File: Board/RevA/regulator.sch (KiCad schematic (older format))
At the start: 0 parts

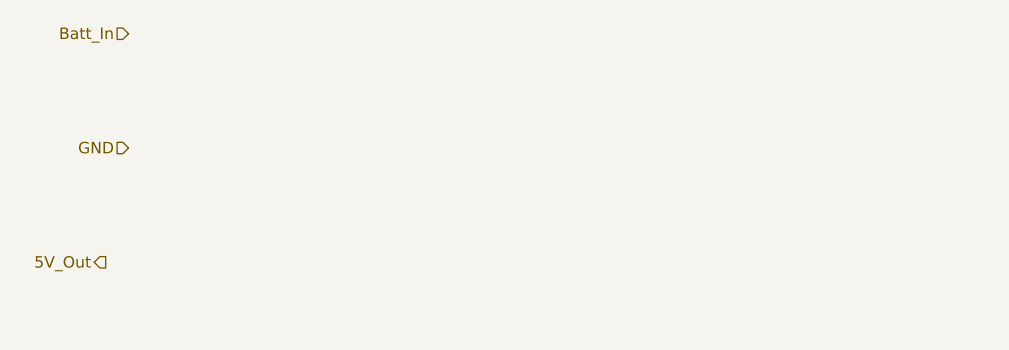
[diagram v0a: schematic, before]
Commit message: Finished Rough RevA and Added Annotations
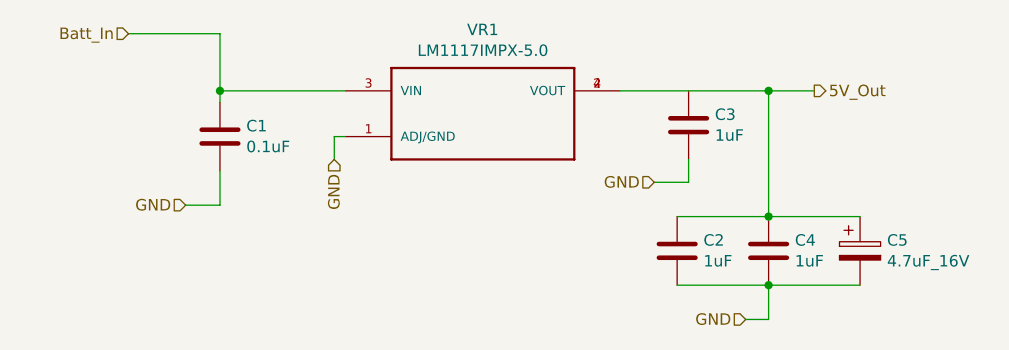
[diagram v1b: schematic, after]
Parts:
- added C1: 0.1uF, symbol Device:C
- added C2, C3, C4: 1uF, symbol Device:C
- added C5: 4.7uF_16V, symbol Device:CP
- added VR1: LM1117IMPX-5.0, symbol LM1117IMPX-5.0:LM1117IMPX-5.0
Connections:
- net 5V_Out: now also C2.1, C4.1, C5.1, VR1.2 (VOUT), VR1.4 (VOUT)
- net Batt_In: now also C1.1, VR1.3 (VIN)
- net GND: now also C1.2, C2.2, C3.2, C4.2, C5.2, VR1.1 (ADJ/GND)
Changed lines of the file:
@@
 Text HLabel 3400 2700 0    50   Input ~ 0
 Batt_In
-Text HLabel 3400 3200 0    50   Input ~ 0
+Text HLabel 3650 3450 0    50   Input ~ 0
 GND
-Text HLabel 3300 3700 0    50   Output ~ 0
+Text HLabel 6400 2950 2    50   Output ~ 0
 5V_Out
+$Comp
+L LM1117IMPX-5.0:LM1117IMPX-5.0 VR1
+U 1 1 614A1D39
+P 4950 3050
+F 0 "VR1" H 4950 3417 50  0000 C CNN
+F 1 "LM1117IMPX-5.0" H 4950 3326 50  0000 C CNN
+F 2 "" H 4950 3050 50  0001 L BNN
+F 3 "1.80 mm" H 4950 3050 50  0001 L BNN
+F 4 "O" H 4950 3050 50  0001 L BNN "Field4"
+F 5 "IPC 7351B" H 4950 3050 50  0001 L BNN "Field5"
+F 6 "Rochester Electronics/Texas Instruments" H 4950 3050 50  0001 L BNN "Field6"
+	1    4950 3050
+	1    0    0    -1
+$EndComp
+$Comp
+L Device:C C1
+U 1 1 614A34B9
+P 3800 3150
+F 0 "C1" H 3915 3196 50  0000 L CNN
+F 1 "0.1uF" H 3915 3105 50  0000 L CNN
+F 2 "" H 3838 3000 50  0001 C CNN
+F 3 "~" H 3800 3150 50  0001 C CNN
+	1    3800 3150
+	1    0    0    -1
+$EndComp
+$Comp
+L Device:C C4
+U 1 1 614A3F1C
+P 6200 3650
+F 0 "C4" H 6315 3696 50  0000 L CNN
+F 1 "1uF" H 6315 3605 50  0000 L CNN
+F 2 "" H 6238 3500 50  0001 C CNN
+F 3 "~" H 6200 3650 50  0001 C CNN
+	1    6200 3650
+	1    0    0    -1
+$EndComp
+Wire Wire Line
+	4350 2950 3800 2950
+Wire Wire Line
+	3800 2950 3800 3000
+Wire Wire Line
+	3800 2950 3800 2700
+Wire Wire Line
+	3800 2700 3400 2700
+Connection ~ 3800 2950
+Wire Wire Line
+	3800 3300 3800 3450
+Wire Wire Line
+	3800 3450 3650 3450
+Wire Wire Line
+	6400 2950 6200 2950
+$Comp
+L Device:C C3
+U 1 1 614A7535
+P 5850 3100
+F 0 "C3" H 5965 3146 50  0000 L CNN
+F 1 "1uF" H 5965 3055 50  0000 L CNN
+F 2 "" H 5888 2950 50  0001 C CNN
+F 3 "~" H 5850 3100 50  0001 C CNN
+	1    5850 3100
+	1    0    0    -1
+$EndComp
+$Comp
+L Device:C C2
+U 1 1 614A7ADA
+P 5800 3650
+F 0 "C2" H 5915 3696 50  0000 L CNN
+F 1 "1uF" H 5915 3605 50  0000 L CNN
+F 2 "" H 5838 3500 50  0001 C CNN
+F 3 "~" H 5800 3650 50  0001 C CNN
+	1    5800 3650
+	1    0    0    -1
+$EndComp
+$Comp
+L Device:CP C5
+U 1 1 614A9413
+P 6600 3650
+F 0 "C5" H 6718 3696 50  0000 L CNN
+F 1 "4.7uF_16V" H 6718 3605 50  0000 L CNN
+F 2 "" H 6638 3500 50  0001 C CNN
+F 3 "~" H 6600 3650 50  0001 C CNN
+	1    6600 3650
+	1    0    0    -1
+$EndComp
+Wire Wire Line
+	6600 3500 6200 3500
+Wire Wire Line
+	6200 3500 5800 3500
+Connection ~ 6200 3500
+Wire Wire Line
+	5800 3800 6200 3800
+Wire Wire Line
+	6600 3800 6200 3800
+Connection ~ 6200 3800
+Wire Wire Line
+	6200 3500 6200 2950
+Connection ~ 6200 2950
+Wire Wire Line
+	6200 2950 5550 2950
+Text HLabel 5700 3350 0    50   Input ~ 0
+GND
+Text HLabel 6100 3950 0    50   Input ~ 0
+GND
+Wire Wire Line
+	6100 3950 6200 3950
+Wire Wire Line
+	6200 3950 6200 3800
+Wire Wire Line
+	5700 3350 5850 3350
+Wire Wire Line
+	5850 3350 5850 3250
+Text HLabel 4300 3250 3    50   Input ~ 0
+GND
+Wire Wire Line
+	4300 3250 4300 3150
+Wire Wire Line
+	4300 3150 4350 3150
 $EndSCHEMATC

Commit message: Added Footprints to RevA 1/2
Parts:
- C1, C2, C3, C4: footprint (none) -> Capacitor_SMD:C_0603_1608Metric
- C5: footprint (none) -> Capacitor_Tantalum_SMD:CP_EIA-3216-18_Kemet-A
- VR1: footprint (none) -> LM1117IMPX-5:SOT230P700X180-4N
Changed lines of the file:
@@
 F 0 "VR1" H 4950 3417 50  0000 C CNN
 F 1 "LM1117IMPX-5.0" H 4950 3326 50  0000 C CNN
-F 2 "" H 4950 3050 50  0001 L BNN
+F 2 "LM1117IMPX-5:SOT230P700X180-4N" H 4950 3050 50  0001 L BNN
 F 3 "1.80 mm" H 4950 3050 50  0001 L BNN
 F 4 "O" H 4950 3050 50  0001 L BNN "Field4"
@@
 F 0 "C1" H 3915 3196 50  0000 L CNN
 F 1 "0.1uF" H 3915 3105 50  0000 L CNN
-F 2 "" H 3838 3000 50  0001 C CNN
+F 2 "Capacitor_SMD:C_0603_1608Metric" H 3838 3000 50  0001 C CNN
 F 3 "~" H 3800 3150 50  0001 C CNN
 	1    3800 3150
@@
 F 0 "C4" H 6315 3696 50  0000 L CNN
 F 1 "1uF" H 6315 3605 50  0000 L CNN
-F 2 "" H 6238 3500 50  0001 C CNN
+F 2 "Capacitor_SMD:C_0603_1608Metric" H 6238 3500 50  0001 C CNN
 F 3 "~" H 6200 3650 50  0001 C CNN
 	1    6200 3650
@@
 F 0 "C3" H 5965 3146 50  0000 L CNN
 F 1 "1uF" H 5965 3055 50  0000 L CNN
-F 2 "" H 5888 2950 50  0001 C CNN
+F 2 "Capacitor_SMD:C_0603_1608Metric" H 5888 2950 50  0001 C CNN
 F 3 "~" H 5850 3100 50  0001 C CNN
 	1    5850 3100
@@
 F 0 "C2" H 5915 3696 50  0000 L CNN
 F 1 "1uF" H 5915 3605 50  0000 L CNN
-F 2 "" H 5838 3500 50  0001 C CNN
+F 2 "Capacitor_SMD:C_0603_1608Metric" H 5838 3500 50  0001 C CNN
 F 3 "~" H 5800 3650 50  0001 C CNN
 	1    5800 3650
@@
 F 0 "C5" H 6718 3696 50  0000 L CNN
 F 1 "4.7uF_16V" H 6718 3605 50  0000 L CNN
-F 2 "" H 6638 3500 50  0001 C CNN
+F 2 "Capacitor_Tantalum_SMD:CP_EIA-3216-18_Kemet-A" H 6638 3500 50  0001 C CNN
 F 3 "~" H 6600 3650 50  0001 C CNN
 	1    6600 3650
